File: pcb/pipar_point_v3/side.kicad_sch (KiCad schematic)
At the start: 19 parts, among them J3 Conn_02x03_Odd_Even, SW1 EVP-BB1AAB000, U1 ISP1807-LR-RS

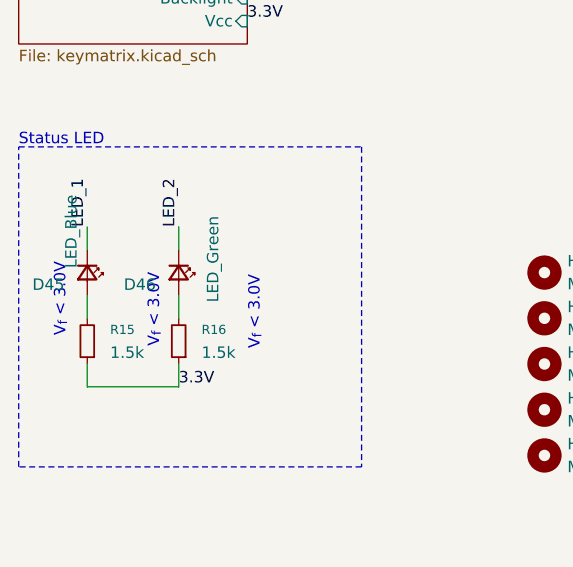
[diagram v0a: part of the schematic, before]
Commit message: Adds trackpoint reset GPIO Fix floating led 15 and 35 (mirrored)
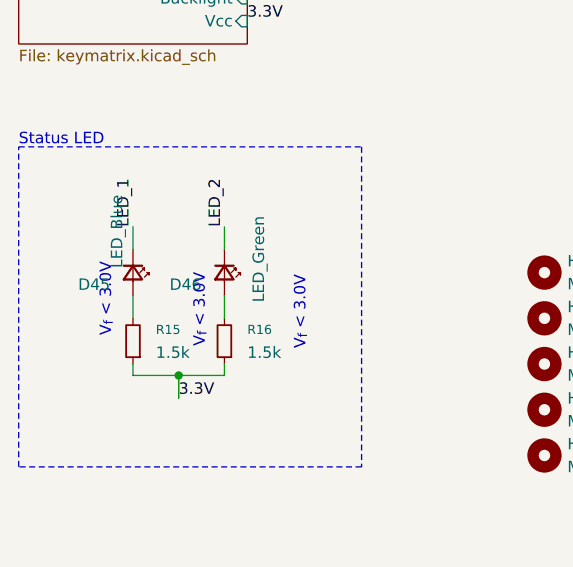
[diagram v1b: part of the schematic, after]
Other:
- moved on the sheet: D45, D46, R15, R16
